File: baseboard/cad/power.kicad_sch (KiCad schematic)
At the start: 39 parts, among them J21 2P_HEADER, J22 2P_HEADER, U7 TLV767, U8 LT3463, U9 LT3032

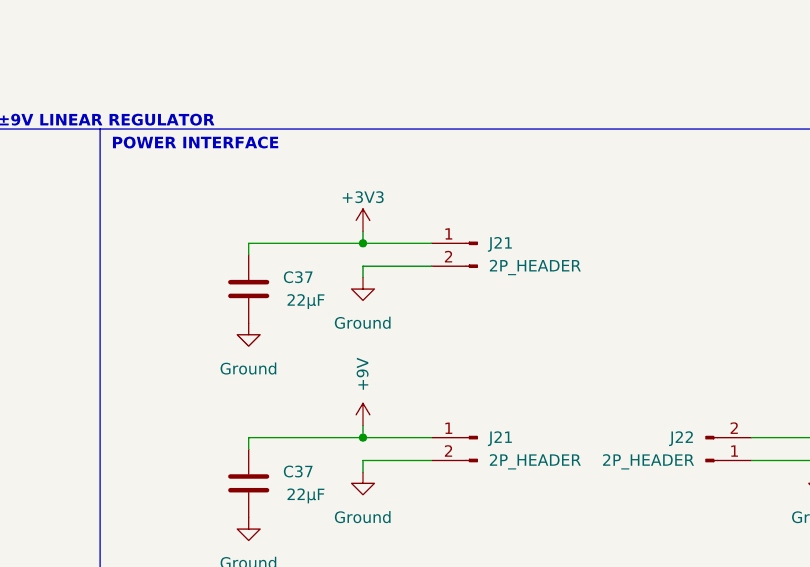
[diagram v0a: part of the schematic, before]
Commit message: finished initial layout
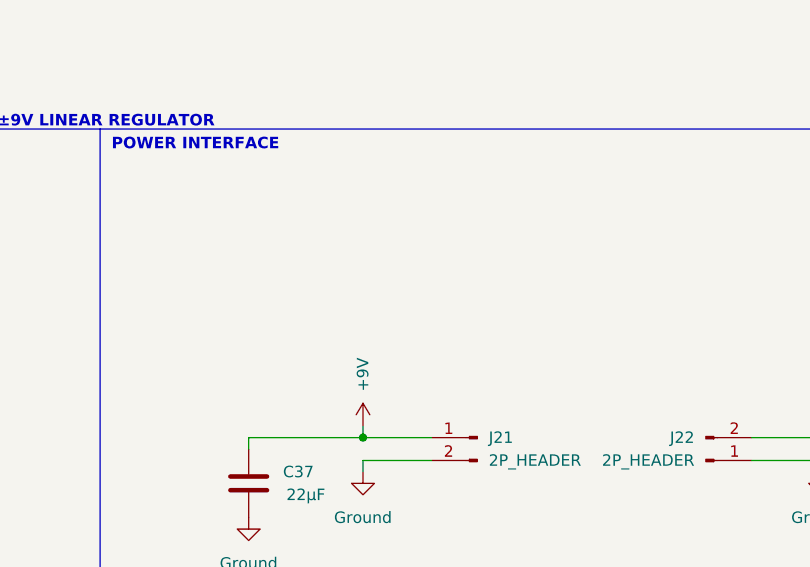
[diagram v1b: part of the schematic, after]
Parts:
- removed C37: 22μF, Capacitor_SMD:C_0805_2012Metric, symbol Device:C
- removed J21: 2P_HEADER, Connector_PinSocket_2.54mm:PinSocket_1x02_P2.54mm_Vertical, symbol Connector:Conn_01x02_Male
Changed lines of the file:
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@@
   (junction (at 57.15 135.89) (diameter 0) (color 0 0 0 0)
   )
-  (junction (at 168.91 114.3) (diameter 0) (color 0 0 0 0)
-  )
   (junction (at 226.06 78.74) (diameter 0) (color 0 0 0 0)
   )
@@
     (stroke (width 0) (type default))
   )
-  (wire (pts (xy 168.91 118.11) (xy 168.91 116.84))
-    (stroke (width 0) (type default))
-  )
   (wire (pts (xy 29.21 48.26) (xy 29.21 49.53))
     (stroke (width 0) (type default))
@@
     (stroke (width 0) (type default))
   )
-  (wire (pts (xy 168.91 114.3) (xy 156.21 114.3))
-    (stroke (width 0) (type default))
-  )
   (wire (pts (xy 158.75 73.66) (xy 160.02 73.66))
     (stroke (width 0) (type default))
@@
     (stroke (width 0) (type default))
   )
-  (wire (pts (xy 168.91 113.03) (xy 168.91 114.3))
-    (stroke (width 0) (type default))
-  )
   (wire (pts (xy 219.71 135.89) (xy 231.14 135.89))
     (stroke (width 0) (type default))
@@
     (stroke (width 0) (type default))
   )
-  (wire (pts (xy 168.91 114.3) (xy 176.53 114.3))
-    (stroke (width 0) (type default))
-  )
   (wire (pts (xy 95.25 53.34) (xy 107.95 53.34))
     (stroke (width 0) (type default))
@@
     (stroke (width 0) (type default))
   )
-  (wire (pts (xy 168.91 116.84) (xy 176.53 116.84))
-    (stroke (width 0) (type default))
-  )
   (wire (pts (xy 107.95 78.74) (xy 115.57 78.74))
     (stroke (width 0) (type default))
@@
   )
   (polyline (pts (xy 25.4 101.6) (xy 254 101.6))
-    (stroke (width 0) (type default))
-  )
-  (wire (pts (xy 156.21 114.3) (xy 156.21 115.57))
     (stroke (width 0) (type default))
   )
@@
         (path "/190888c1-6ce2-4681-a836-dc477e444e49/2e4f7641-7de0-4dea-9f64-f5ec09624375"
           (reference "D6") (unit 1)
-        )
-      )
-    )
-  )
-  (symbol (lib_id "Library:Ground") (at 168.91 118.11 0) (unit 1)
-    (in_bom yes) (on_board yes) (dnp no)
-    (property "Reference" "#PWR056" (at 168.91 124.46 0)
-      (effects (font (size 1.27 1.27)) hide)
-    )
-    (property "Value" "Ground" (at 168.91 123.19 0)
-      (effects (font (size 1.27 1.27)))
-    )
-    (property "Footprint" "" (at 168.91 118.11 0)
-      (effects (font (size 1.27 1.27)) hide)
-    )
-    (property "Datasheet" "" (at 168.91 118.11 0)
-      (effects (font (size 1.27 1.27)) hide)
-    )
-    (pin "1")
-    (instances
-      (project "1590N1 IO Board"
-        (path "/190888c1-6ce2-4681-a836-dc477e444e49/229a97b2-4425-47f7-b588-f32dc6b9bc79"
-          (reference "#PWR056") (unit 1)
-        )
-        (path "/190888c1-6ce2-4681-a836-dc477e444e49/e436358c-d730-4540-92b5-b7475a7c4a63"
-          (reference "#PWR047") (unit 1)
-        )
-        (path "/190888c1-6ce2-4681-a836-dc477e444e49/2e4f7641-7de0-4dea-9f64-f5ec09624375"
-          (reference "#PWR052") (unit 1)
         )
       )
@@
     )
   )
-  (symbol (lib_id "power:+3V3") (at 168.91 113.03 0) (unit 1)
-    (in_bom yes) (on_board yes) (dnp no) (fields_autoplaced)
-    (property "Reference" "#PWR047" (at 168.91 116.84 0)
-      (effects (font (size 1.27 1.27)) hide)
-    )
-    (property "Value" "+3V3" (at 168.91 109.22 0)
-      (effects (font (size 1.27 1.27)))
-    )
-    (property "Footprint" "" (at 168.91 113.03 0)
-      (effects (font (size 1.27 1.27)) hide)
-    )
-    (property "Datasheet" "" (at 168.91 113.03 0)
-      (effects (font (size 1.27 1.27)) hide)
-    )
-    (pin "1")
-    (instances
-      (project "1590N1 IO Board"
-        (path "/190888c1-6ce2-4681-a836-dc477e444e49/2e4f7641-7de0-4dea-9f64-f5ec09624375"
-          (reference "#PWR047") (unit 1)
-        )
-      )
-    )
-  )
   (symbol (lib_id "Device:C") (at 231.14 140.97 180) (unit 1)
     (in_bom yes) (on_board yes) (dnp no)
@@
         (path "/190888c1-6ce2-4681-a836-dc477e444e49/2e4f7641-7de0-4dea-9f64-f5ec09624375"
           (reference "#FLG04") (unit 1)
-        )
-      )
-    )
-  )
-  (symbol (lib_id "Device:C") (at 156.21 119.38 180) (unit 1)
-    (in_bom yes) (on_board yes) (dnp no)
-    (property "Reference" "C37" (at 160.02 118.11 0)
-      (effects (font (size 1.27 1.27)) (justify right))
-    )
-    (property "Value" "22μF" (at 162.56 120.65 0)
-      (effects (font (size 1.27 1.27)))
-    )
-    (property "Footprint" "Capacitor_SMD:C_0805_2012Metric" (at 155.2448 115.57 0)
-      (effects (font (size 1.27 1.27)) hide)
-    )
-    (property "Datasheet" "https://www.murata.com/en-us/products/capacitor/ceramiccapacitor/overview/lineup/smd/grm#anchor-2" (at 156.21 119.38 0)
-      (effects (font (size 1.27 1.27)) hide)
-    )
-    (property "Manufacturer" "Murata" (at 156.21 119.38 0)
-      (effects (font (size 1.27 1.27)) hide)
-    )
-    (property "Part Number" "GRM21BR61E226ME44L" (at 156.21 119.38 0)
-      (effects (font (size 1.27 1.27)) hide)
-    )
-    (pin "1")
-    (pin "2")
-    (instances
-      (project "1590N1 IO Board"
-        (path "/190888c1-6ce2-4681-a836-dc477e444e49/229a97b2-4425-47f7-b588-f32dc6b9bc79"
-          (reference "C37") (unit 1)
-        )
-        (path "/190888c1-6ce2-4681-a836-dc477e444e49/e436358c-d730-4540-92b5-b7475a7c4a63"
-          (reference "C33") (unit 1)
-        )
-        (path "/190888c1-6ce2-4681-a836-dc477e444e49/2e4f7641-7de0-4dea-9f64-f5ec09624375"
-          (reference "C37") (unit 1)
         )
       )
@@
     )
   )
-  (symbol (lib_id "Library:Ground") (at 156.21 123.19 0) (unit 1)
-    (in_bom yes) (on_board yes) (dnp no)
-    (property "Reference" "#PWR047" (at 156.21 129.54 0)
-      (effects (font (size 1.27 1.27)) hide)
-    )
-    (property "Value" "Ground" (at 156.21 128.27 0)
-      (effects (font (size 1.27 1.27)))
-    )
-    (property "Footprint" "" (at 156.21 123.19 0)
-      (effects (font (size 1.27 1.27)) hide)
-    )
-    (property "Datasheet" "" (at 156.21 123.19 0)
-      (effects (font (size 1.27 1.27)) hide)
-    )
-    (pin "1")
-    (instances
-      (project "1590N1 IO Board"
-        (path "/190888c1-6ce2-4681-a836-dc477e444e49/229a97b2-4425-47f7-b588-f32dc6b9bc79"
-          (reference "#PWR047") (unit 1)
-        )
-        (path "/190888c1-6ce2-4681-a836-dc477e444e49/e436358c-d730-4540-92b5-b7475a7c4a63"
-          (reference "#PWR045") (unit 1)
-        )
-        (path "/190888c1-6ce2-4681-a836-dc477e444e49/2e4f7641-7de0-4dea-9f64-f5ec09624375"
-          (reference "#PWR046") (unit 1)
-        )
-      )
-    )
-  )
   (symbol (lib_id "Library:Ground") (at 140.97 59.69 0) (unit 1)
     (in_bom yes) (on_board yes) (dnp no)
@@
         )
       )
-    )
-  )
-  (symbol (lib_id "Connector:Conn_01x02_Male") (at 181.61 114.3 0) (mirror y) (unit 1)
-    (in_bom yes) (on_board yes) (dnp no) (fields_autoplaced)
-    (property "Reference" "J21" (at 182.88 114.2999 0)
-      (effects (font (size 1.27 1.27)) (justify right))
-    )
-    (property "Value" "2P_HEADER" (at 182.88 116.8399 0)
-      (effects (font (size 1.27 1.27)) (justify right))
-    )
-    (property "Footprint" "Connector_PinSocket_2.54mm:PinSocket_1x02_P2.54mm_Vertical" (at 181.61 114.3 0)
-      (effects (font (size 1.27 1.27)) hide)
-    )
-    (property "Datasheet" "~" (at 181.61 114.3 0)
-      (effects (font (size 1.27 1.27)) hide)
-    )
-    (property "Manufacturer" "Samtec" (at 181.61 114.3 0)
-      (effects (font (size 1.27 1.27)) hide)
-    )
-    (pin "1")
-    (pin "2")
-    (instances
-      (project "1590N1 IO Board"
-        (path "/190888c1-6ce2-4681-a836-dc477e444e49/229a97b2-4425-47f7-b588-f32dc6b9bc79"
-          (reference "J21") (unit 1)
-        )
-        (path "/190888c1-6ce2-4681-a836-dc477e444e49/e436358c-d730-4540-92b5-b7475a7c4a63"
-          (reference "J21") (unit 1)
-        )
-        (path "/190888c1-6ce2-4681-a836-dc477e444e49/2e4f7641-7de0-4dea-9f64-f5ec09624375"
-          (reference "J8") (unit 1)
-        )
-      )

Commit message: more early layout work
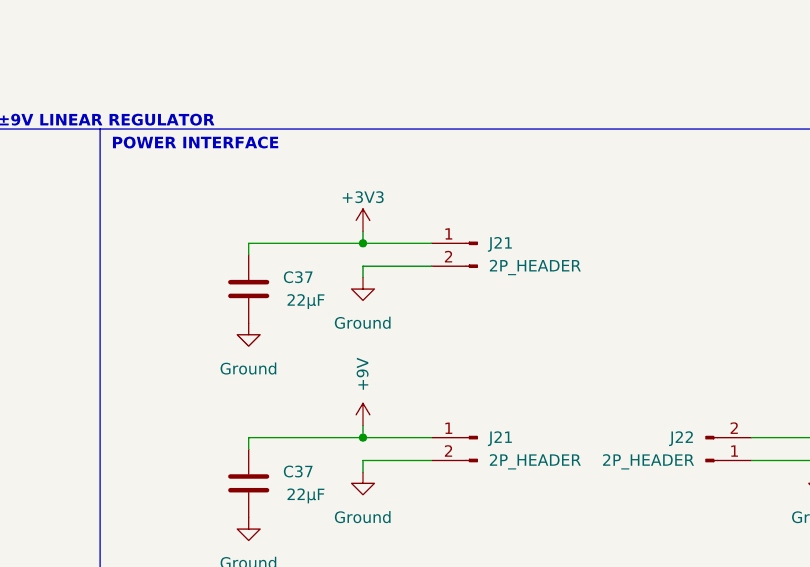
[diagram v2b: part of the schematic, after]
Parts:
- added C37: 22μF, Capacitor_SMD:C_0805_2012Metric, symbol Device:C
- added J21: 2P_HEADER, Connector_PinSocket_2.54mm:PinSocket_1x02_P2.54mm_Vertical, symbol Connector:Conn_01x02_Male
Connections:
- net +3V3: now also C37.2, J21.1 (Pin_1)
- net GND: now also C37.1, J21.2 (Pin_2)
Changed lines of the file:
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@@
   (junction (at 57.15 135.89) (diameter 0) (color 0 0 0 0)
   )
+  (junction (at 168.91 114.3) (diameter 0) (color 0 0 0 0)
+  )
   (junction (at 226.06 78.74) (diameter 0) (color 0 0 0 0)
   )
@@
     (stroke (width 0) (type default))
   )
+  (wire (pts (xy 168.91 118.11) (xy 168.91 116.84))
+    (stroke (width 0) (type default))
+  )
   (wire (pts (xy 29.21 48.26) (xy 29.21 49.53))
     (stroke (width 0) (type default))
@@
     (stroke (width 0) (type default))
   )
+  (wire (pts (xy 168.91 114.3) (xy 156.21 114.3))
+    (stroke (width 0) (type default))
+  )
   (wire (pts (xy 158.75 73.66) (xy 160.02 73.66))
     (stroke (width 0) (type default))
@@
     (stroke (width 0) (type default))
   )
+  (wire (pts (xy 168.91 113.03) (xy 168.91 114.3))
+    (stroke (width 0) (type default))
+  )
   (wire (pts (xy 219.71 135.89) (xy 231.14 135.89))
     (stroke (width 0) (type default))
@@
     (stroke (width 0) (type default))
   )
+  (wire (pts (xy 168.91 114.3) (xy 176.53 114.3))
+    (stroke (width 0) (type default))
+  )
   (wire (pts (xy 95.25 53.34) (xy 107.95 53.34))
     (stroke (width 0) (type default))
@@
     (stroke (width 0) (type default))
   )
+  (wire (pts (xy 168.91 116.84) (xy 176.53 116.84))
+    (stroke (width 0) (type default))
+  )
   (wire (pts (xy 107.95 78.74) (xy 115.57 78.74))
     (stroke (width 0) (type default))
@@
   )
   (polyline (pts (xy 25.4 101.6) (xy 254 101.6))
+    (stroke (width 0) (type default))
+  )
+  (wire (pts (xy 156.21 114.3) (xy 156.21 115.57))
     (stroke (width 0) (type default))
   )
@@
         (path "/190888c1-6ce2-4681-a836-dc477e444e49/2e4f7641-7de0-4dea-9f64-f5ec09624375"
           (reference "D6") (unit 1)
+        )
+      )
+    )
+  )
+  (symbol (lib_id "Library:Ground") (at 168.91 118.11 0) (unit 1)
+    (in_bom yes) (on_board yes) (dnp no)
+    (property "Reference" "#PWR056" (at 168.91 124.46 0)
+      (effects (font (size 1.27 1.27)) hide)
+    )
+    (property "Value" "Ground" (at 168.91 123.19 0)
+      (effects (font (size 1.27 1.27)))
+    )
+    (property "Footprint" "" (at 168.91 118.11 0)
+      (effects (font (size 1.27 1.27)) hide)
+    )
+    (property "Datasheet" "" (at 168.91 118.11 0)
+      (effects (font (size 1.27 1.27)) hide)
+    )
+    (pin "1")
+    (instances
+      (project "1590N1 IO Board"
+        (path "/190888c1-6ce2-4681-a836-dc477e444e49/229a97b2-4425-47f7-b588-f32dc6b9bc79"
+          (reference "#PWR056") (unit 1)
+        )
+        (path "/190888c1-6ce2-4681-a836-dc477e444e49/e436358c-d730-4540-92b5-b7475a7c4a63"
+          (reference "#PWR047") (unit 1)
+        )
+        (path "/190888c1-6ce2-4681-a836-dc477e444e49/2e4f7641-7de0-4dea-9f64-f5ec09624375"
+          (reference "#PWR052") (unit 1)
         )
       )
@@
     )
   )
+  (symbol (lib_id "power:+3V3") (at 168.91 113.03 0) (unit 1)
+    (in_bom yes) (on_board yes) (dnp no) (fields_autoplaced)
+    (property "Reference" "#PWR047" (at 168.91 116.84 0)
+      (effects (font (size 1.27 1.27)) hide)
+    )
+    (property "Value" "+3V3" (at 168.91 109.22 0)
+      (effects (font (size 1.27 1.27)))
+    )
+    (property "Footprint" "" (at 168.91 113.03 0)
+      (effects (font (size 1.27 1.27)) hide)
+    )
+    (property "Datasheet" "" (at 168.91 113.03 0)
+      (effects (font (size 1.27 1.27)) hide)
+    )
+    (pin "1")
+    (instances
+      (project "1590N1 IO Board"
+        (path "/190888c1-6ce2-4681-a836-dc477e444e49/2e4f7641-7de0-4dea-9f64-f5ec09624375"
+          (reference "#PWR047") (unit 1)
+        )
+      )
+    )
+  )
   (symbol (lib_id "Device:C") (at 231.14 140.97 180) (unit 1)
     (in_bom yes) (on_board yes) (dnp no)
@@
         (path "/190888c1-6ce2-4681-a836-dc477e444e49/2e4f7641-7de0-4dea-9f64-f5ec09624375"
           (reference "#FLG04") (unit 1)
+        )
+      )
+    )
+  )
+  (symbol (lib_id "Device:C") (at 156.21 119.38 180) (unit 1)
+    (in_bom yes) (on_board yes) (dnp no)
+    (property "Reference" "C37" (at 160.02 118.11 0)
+      (effects (font (size 1.27 1.27)) (justify right))
+    )
+    (property "Value" "22μF" (at 162.56 120.65 0)
+      (effects (font (size 1.27 1.27)))
+    )
+    (property "Footprint" "Capacitor_SMD:C_0805_2012Metric" (at 155.2448 115.57 0)
+      (effects (font (size 1.27 1.27)) hide)
+    )
+    (property "Datasheet" "https://www.murata.com/en-us/products/capacitor/ceramiccapacitor/overview/lineup/smd/grm#anchor-2" (at 156.21 119.38 0)
+      (effects (font (size 1.27 1.27)) hide)
+    )
+    (property "Manufacturer" "Murata" (at 156.21 119.38 0)
+      (effects (font (size 1.27 1.27)) hide)
+    )
+    (property "Part Number" "GRM21BR61E226ME44L" (at 156.21 119.38 0)
+      (effects (font (size 1.27 1.27)) hide)
+    )
+    (pin "1")
+    (pin "2")
+    (instances
+      (project "1590N1 IO Board"
+        (path "/190888c1-6ce2-4681-a836-dc477e444e49/229a97b2-4425-47f7-b588-f32dc6b9bc79"
+          (reference "C37") (unit 1)
+        )
+        (path "/190888c1-6ce2-4681-a836-dc477e444e49/e436358c-d730-4540-92b5-b7475a7c4a63"
+          (reference "C33") (unit 1)
+        )
+        (path "/190888c1-6ce2-4681-a836-dc477e444e49/2e4f7641-7de0-4dea-9f64-f5ec09624375"
+          (reference "C37") (unit 1)
         )
       )
@@
     )
   )
+  (symbol (lib_id "Library:Ground") (at 156.21 123.19 0) (unit 1)
+    (in_bom yes) (on_board yes) (dnp no)
+    (property "Reference" "#PWR047" (at 156.21 129.54 0)
+      (effects (font (size 1.27 1.27)) hide)
+    )
+    (property "Value" "Ground" (at 156.21 128.27 0)
+      (effects (font (size 1.27 1.27)))
+    )
+    (property "Footprint" "" (at 156.21 123.19 0)
+      (effects (font (size 1.27 1.27)) hide)
+    )
+    (property "Datasheet" "" (at 156.21 123.19 0)
+      (effects (font (size 1.27 1.27)) hide)
+    )
+    (pin "1")
+    (instances
+      (project "1590N1 IO Board"
+        (path "/190888c1-6ce2-4681-a836-dc477e444e49/229a97b2-4425-47f7-b588-f32dc6b9bc79"
+          (reference "#PWR047") (unit 1)
+        )
+        (path "/190888c1-6ce2-4681-a836-dc477e444e49/e436358c-d730-4540-92b5-b7475a7c4a63"
+          (reference "#PWR045") (unit 1)
+        )
+        (path "/190888c1-6ce2-4681-a836-dc477e444e49/2e4f7641-7de0-4dea-9f64-f5ec09624375"
+          (reference "#PWR046") (unit 1)
+        )
+      )
+    )
+  )
   (symbol (lib_id "Library:Ground") (at 140.97 59.69 0) (unit 1)
     (in_bom yes) (on_board yes) (dnp no)
@@
         )
       )
+    )
+  )
+  (symbol (lib_id "Connector:Conn_01x02_Male") (at 181.61 114.3 0) (mirror y) (unit 1)
+    (in_bom yes) (on_board yes) (dnp no) (fields_autoplaced)
+    (property "Reference" "J21" (at 182.88 114.2999 0)
+      (effects (font (size 1.27 1.27)) (justify right))
+    )
+    (property "Value" "2P_HEADER" (at 182.88 116.8399 0)
+      (effects (font (size 1.27 1.27)) (justify right))
+    )
+    (property "Footprint" "Connector_PinSocket_2.54mm:PinSocket_1x02_P2.54mm_Vertical" (at 181.61 114.3 0)
+      (effects (font (size 1.27 1.27)) hide)
+    )
+    (property "Datasheet" "~" (at 181.61 114.3 0)
+      (effects (font (size 1.27 1.27)) hide)
+    )
+    (property "Manufacturer" "Samtec" (at 181.61 114.3 0)
+      (effects (font (size 1.27 1.27)) hide)
+    )
+    (pin "1")
+    (pin "2")
+    (instances
+      (project "1590N1 IO Board"
+        (path "/190888c1-6ce2-4681-a836-dc477e444e49/229a97b2-4425-47f7-b588-f32dc6b9bc79"
+          (reference "J21") (unit 1)
+        )
+        (path "/190888c1-6ce2-4681-a836-dc477e444e49/e436358c-d730-4540-92b5-b7475a7c4a63"
+          (reference "J21") (unit 1)
+        )
+        (path "/190888c1-6ce2-4681-a836-dc477e444e49/2e4f7641-7de0-4dea-9f64-f5ec09624375"
+          (reference "J8") (unit 1)
+        )
+      )
